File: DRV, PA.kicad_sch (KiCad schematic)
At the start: 26 parts, among them Q1 2SC5171, Q2 2SA1930, Q3 IRF630, Q4 IRF630

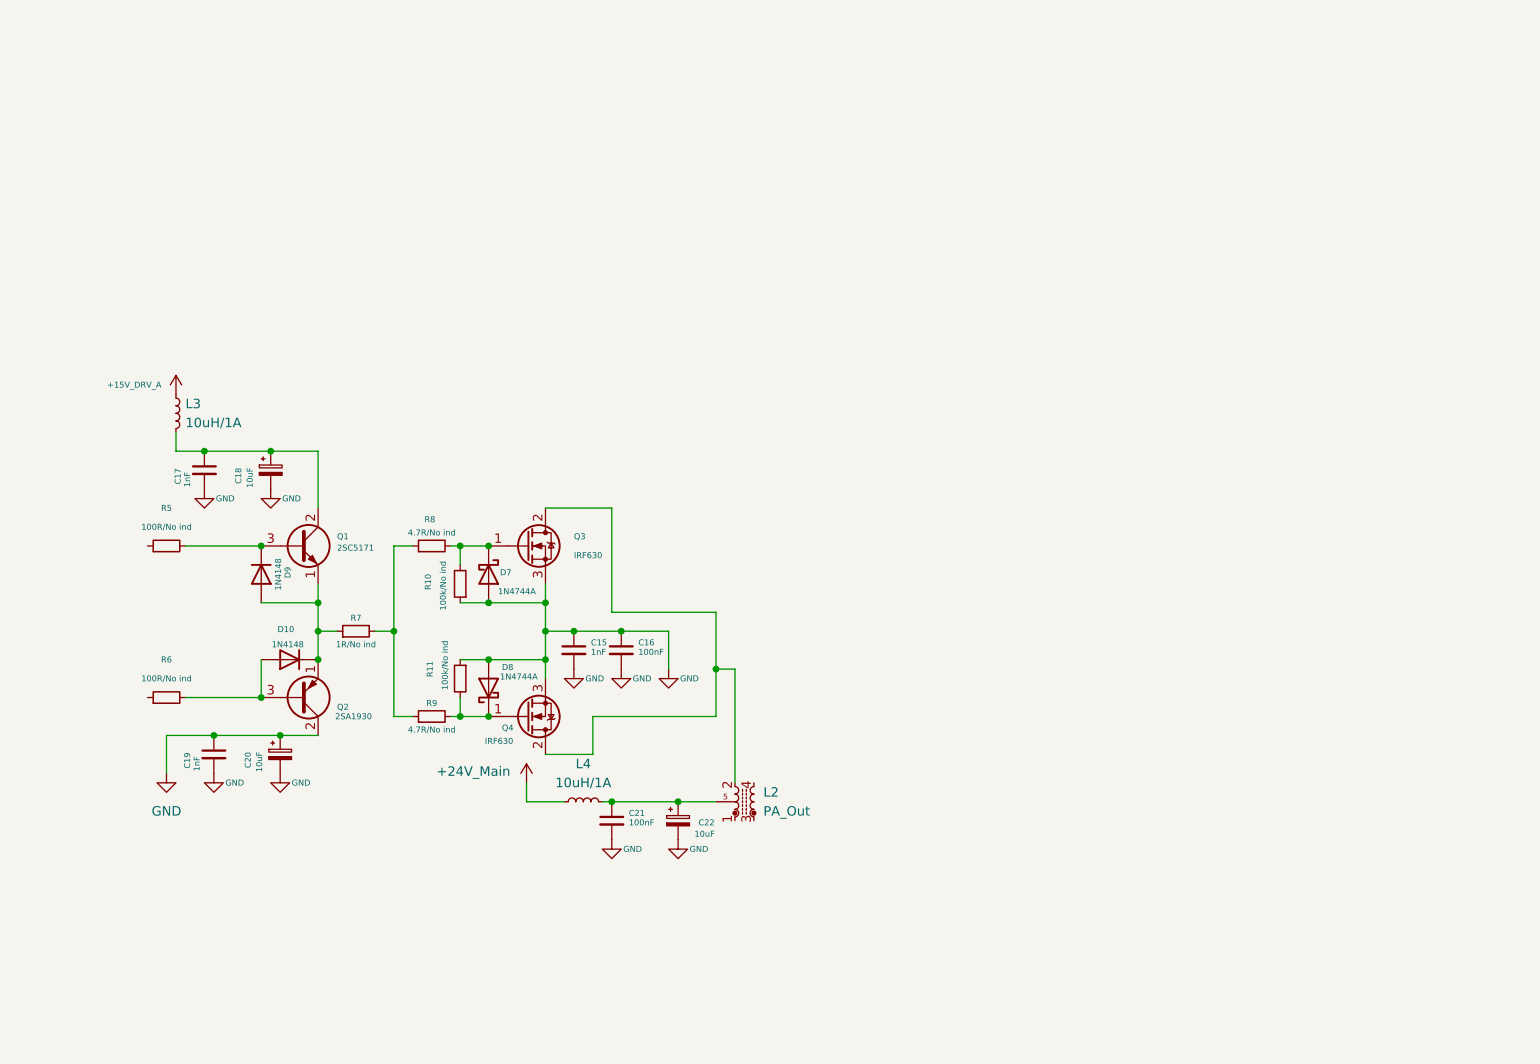
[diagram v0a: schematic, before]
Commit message: Bias Work
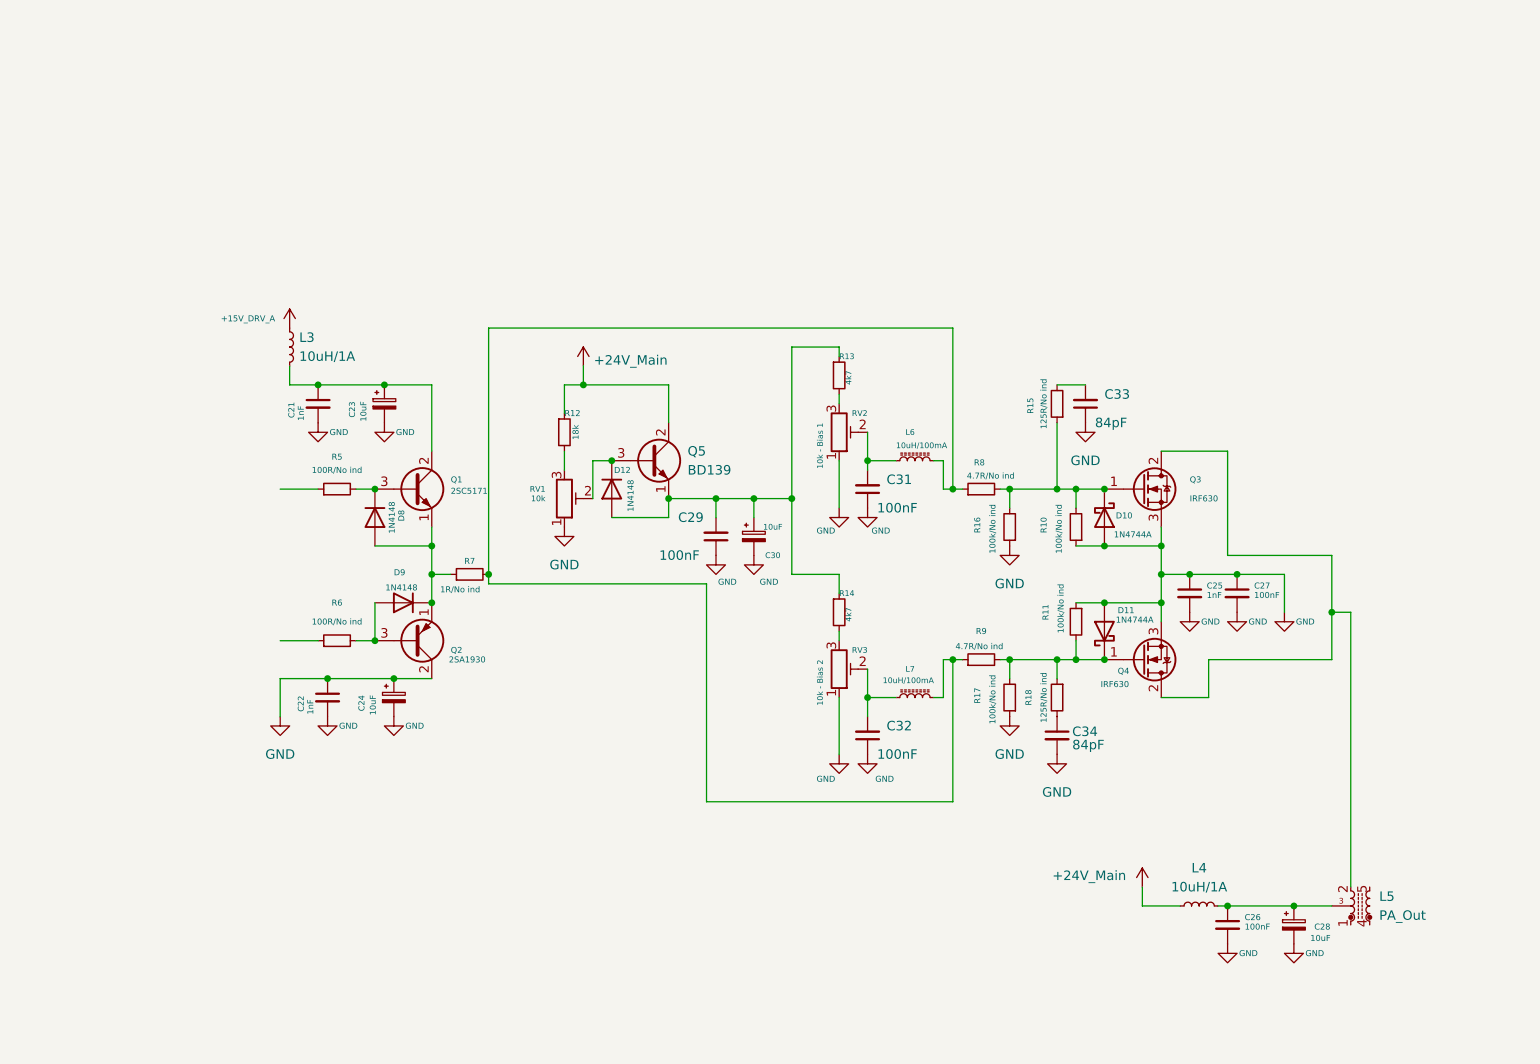
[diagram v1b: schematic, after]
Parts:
- removed L2: PA_Out, symbol Intralha.:L_Ferrite_Taped_Coupled_Small_2
- added C29, C31, C32: 100nF, symbol Device:C_Small
- added C30: 10uF, symbol Device:C_Polarized_Small
- added C33, C34: 84pF, symbol Device:C_Small
- added D12: 1N4148, Diode_THT:D_DO-35_SOD27_P7.62mm_Horizontal, symbol Diode:1N4148
- added L5: PA_Out, symbol Intralha.:L_Ferrite_Taped_Coupled_Small_2
- added L6, L7: 10uH/100mA, symbol Device:L_Ferrite_Small
- added Q5: BD139, Package_TO_SOT_THT:TO-126-3_Vertical, symbol Transistor_BJT:BD139
- added R12: 18k, symbol Device:R_Small
- added R13, R14: 4k7, symbol Device:R_Small
- added R15, R18: 125R/No ind, symbol Device:R_Small
- added R16, R17: 100k/No ind, symbol Device:R_Small
- added RV1: 10k, symbol Device:R_Potentiometer_Trim
- added RV2: 10k - Bias 1, symbol Device:R_Potentiometer_Trim
- added RV3: 10k - Bias 2, symbol Device:R_Potentiometer_Trim
- renumbered C17 to C21, C19 to C22, C18 to C23, C20 to C24, C15 to C25, C21 to C26, C16 to C27, C22 to C28, D7 to D10, D8 to D11, D9 to D8, D10 to D9
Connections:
- net +24V_Main: now also Q5.2 (C), R12.1
- net GND: now also C29.1, C30.2, C31.1, C32.1, C33.1, C34.2, R16.1, R17.1, RV1.1, RV2.1, RV3.1
- net at R7.2, R8.1, R9.1: now also L6.2, L7.2
- net at D11.1 (K), Q4.1 (G), R11.2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: now also R17.2, R18.1
- net at Q3.2 (D), Q4.2 (D): now also L5.2
- net at D10.1 (K), Q3.1 (G), R10.2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: now also R15.1, R16.2
- net at C26.1, C28.1, L4.2: now also L5.3 (Tap)
- new net: C33.2, R15.2
- new net: C29.2, C30.1, D12.2 (A), Q5.1 (E), R13.1, R14.1
- new net: R14.2, RV3.3
- new net: C31.2, L6.1, RV2.2
- new net: C32.2, L7.1, RV3.2
- new net: R13.2, RV2.3
- new net: C34.1, R18.2
- new net: D12.1 (K), Q5.3 (B), RV1.2
- new net: R12.2, RV1.3
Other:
- moved on the sheet: C21, C22, C23, C24, C25, C26, C27, C28, D10, D11, D8, D9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

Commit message: Driver bias
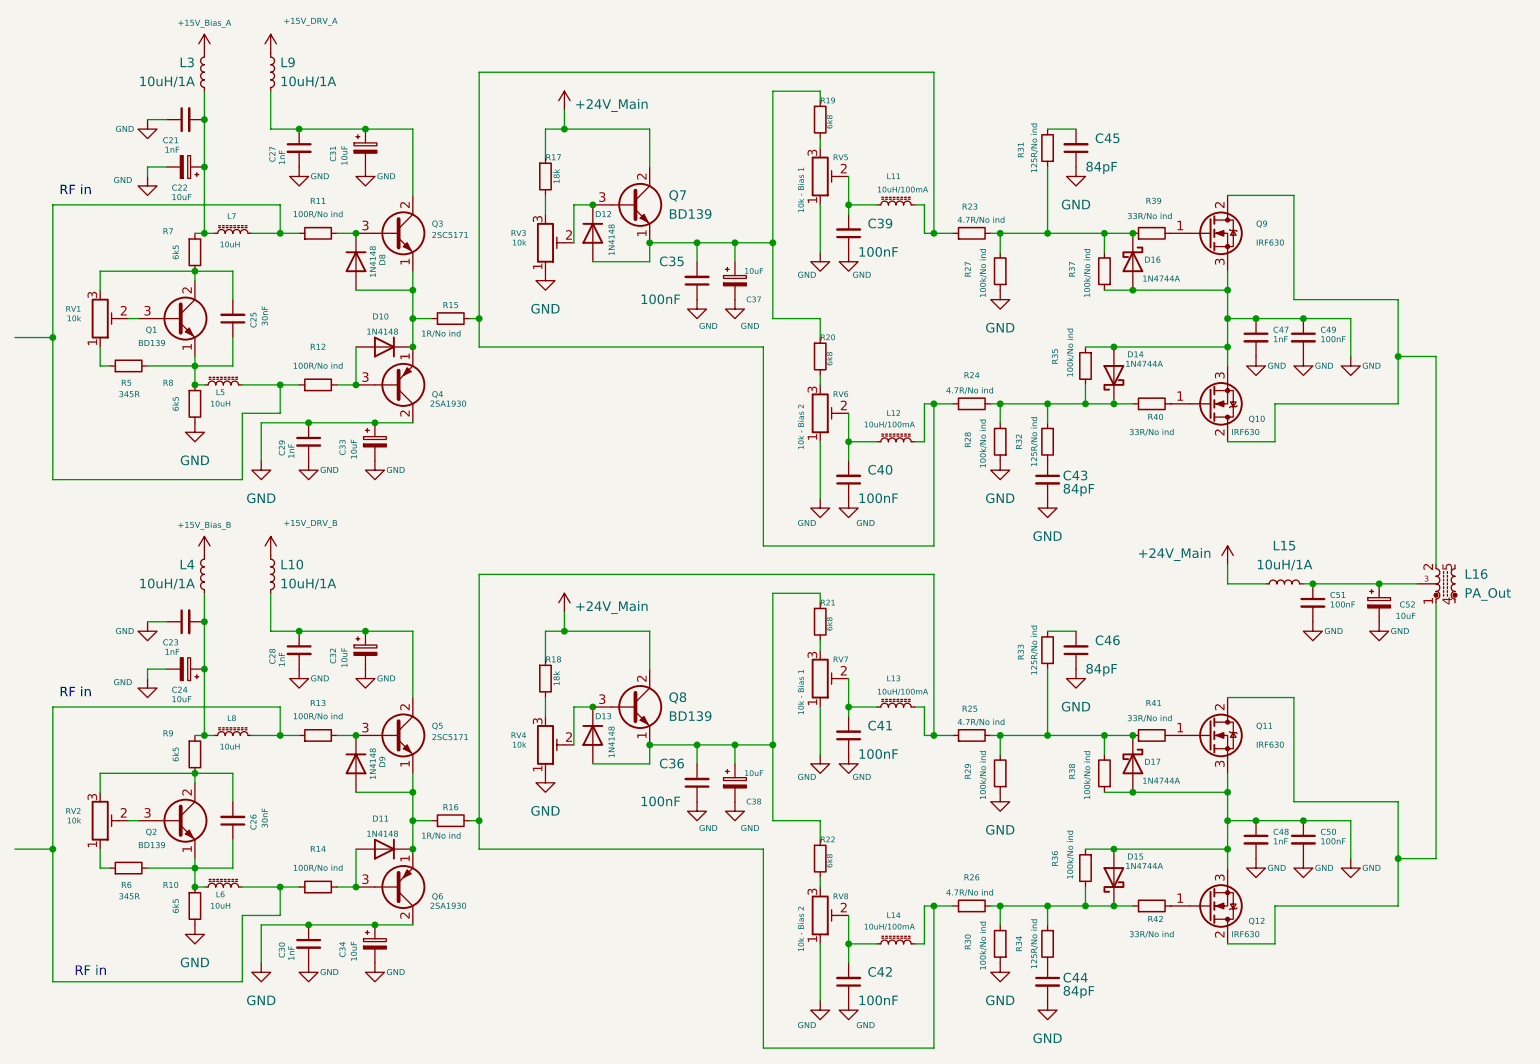
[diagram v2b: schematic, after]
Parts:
- added C21, C23, C28, C30, C48: 1nF, symbol Device:C_Small
- added C22, C24, C32, C34, C38: 10uF, symbol Device:C_Polarized_Small
- added C25, C26: 30nF, symbol Device:C_Small
- added C36, C41, C42, C50: 100nF, symbol Device:C_Small
- added C44, C46: 84pF, symbol Device:C_Small
- added D11, D13, D9: 1N4148, Diode_THT:D_DO-35_SOD27_P7.62mm_Horizontal, symbol Diode:1N4148
- added D15, D17: 1N4744A, symbol Device:D_Schottky
- added L10, L3, L4: 10uH/1A, symbol Device:L_Small
- added L13, L14: 10uH/100mA, symbol Device:L_Ferrite_Small
- added L5, L6, L7, L8: 10uH, symbol Device:L_Ferrite_Small
- added Q1, Q2, Q8: BD139, Package_TO_SOT_THT:TO-126-3_Vertical, symbol Transistor_BJT:BD139
- added Q11, Q12: IRF630, Package_TO_SOT_THT:TO-220-3_Vertical, symbol Transistor_FET:IRF540N
- added Q5: 2SC5171, Package_TO_SOT_THT:TO-126-3_Vertical, symbol Transistor_BJT:BD139
- added Q6: 2SA1930, Package_TO_SOT_THT:TO-126-3_Vertical, symbol Transistor_BJT:BD140
- added R10, R7, R8, R9: 6k5, symbol Device:R_Small
- added R13, R14: 100R/No ind, symbol Device:R_Small
- added R16: 1R/No ind, symbol Device:R_Small
- added R18: 18k, symbol Device:R_Small
- added R21, R22: 6k8, symbol Device:R_Small
- added R25, R26: 4.7R/No ind, symbol Device:R_Small
- added R29, R30, R36, R38: 100k/No ind, symbol Device:R_Small
- added R33, R34: 125R/No ind, symbol Device:R_Small
- added R39, R40, R41, R42: 33R/No ind, symbol Device:R_Small
- added R5, R6: 345R, symbol Device:R_Small
- added RV1, RV2, RV4: 10k, symbol Device:R_Potentiometer_Trim
- added RV7: 10k - Bias 1, symbol Device:R_Potentiometer_Trim
- added RV8: 10k - Bias 2, symbol Device:R_Potentiometer_Trim
- R19: renamed from R13; value 4k7 -> 6k8
- R20: renamed from R14; value 4k7 -> 6k8
- renumbered C21 to C27, C22 to C29, C23 to C31, C24 to C33, C29 to C35, C30 to C37, C31 to C39, C32 to C40, C34 to C43, C33 to C45, C25 to C47, C27 to C49, C26 to C51, C28 to C52, D9 to D10, D11 to D14, D10 to D16, L6 to L11, L7 to L12, L4 to L15, L5 to L16, L3 to L9, Q4 to Q10, Q1 to Q3, Q2 to Q4, Q5 to Q7, Q3 to Q9, R5 to R11, R6 to R12, R7 to R15, R12 to R17, R8 to R23, R9 to R24, R16 to R27, R17 to R28, R15 to R31, R18 to R32, R11 to R35, R10 to R37, RV1 to RV3, RV2 to RV5, RV3 to RV6
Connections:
- net +24V_Main: now also Q8.2 (C), R18.1
- net GND: now also C21.1, C22.2, C23.1, C24.2, C28.2, C30.1, C30.2, C32.2, C34.1, C34.2, C36.1, C38.2, C41.1, C42.1, C44.2, C46.1, C48.1, C48.2, C50.1, C50.2, D15.2 (A), D17.2 (A), Q11.3 (S), Q12.3 (S), Q6.2 (C), R10.2, R29.1, R30.1, R36.1, R38.1, R8.2, RV4.1, RV7.1, RV8.1
- net at D16.1 (K), R23.2, R27.2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: now also R39.1; no longer Q9.1 (G)
- net at D14.1 (K), R24.2, R28.2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: now also R40.1; no longer Q10.1 (G)
- net at L16.1: now also Q11.2 (D), Q12.2 (D)
- net at R11.1: now also R12.1, L5.2, L7.2
- new net: C25.1, L5.1, Q1.1 (E), R5.2, R8.1
- new net: C25.2, Q1.2 (C), R7.2, RV1.3
- new net: D17.1 (K), R25.2, R29.2, R33.1, R38.2, R41.1
- new net: C46.2, R33.2
- new net: R6.1, RV2.1
- new net: C26.1, L6.1, Q2.1 (E), R10.1, R6.2
- new net: L6.2, L8.2, R13.1, R14.1
- new net: D9.1 (K), Q5.3 (B), R13.2
- new net: D11.1 (K), D9.2 (A), Q5.1 (E), Q6.1 (E), R16.1
- new net: L13.2, L14.2, R16.2, R25.1, R26.1
- new net: C42.2, L14.1, RV8.2
- new net: C28.1, C32.1, L10.2, Q5.2 (C)
- new net: R5.1, RV1.1
- new net: Q1.3 (B), RV1.2
- new net: C26.2, Q2.2 (C), R9.2, RV2.3
- new net: Q2.3 (B), RV2.2
- new net: C44.1, R34.2
- new net: C23.2, C24.1, L4.2, L8.1, R9.1
- new net: D13.1 (K), Q8.3 (B), RV4.2
- new net: R18.2, RV4.3
- new net: D15.1 (K), R26.2, R30.2, R34.1, R36.2, R42.1
- new net: Q12.1 (G), R42.2
- new net: C21.2, C22.1, L3.2, L7.1, R7.1
- new net: R22.2, RV8.3
- new net: Q11.1 (G), R41.2
- new net: Q10.1 (G), R40.2
- new net: C36.2, C38.1, D13.2 (A), Q8.1 (E), R21.1, R22.1
- new net: C41.2, L13.1, RV7.2
- new net: R21.2, RV7.3
- new net: Q9.1 (G), R39.2
- new net: D11.2 (A), Q6.3 (B), R14.2
- new net +15V_Bias_A: L3.1
- new net +15V_Bias_B: L4.1
- new net +15V_DRV_B: L10.1
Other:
- note added: "RF in"
- moved on the sheet: C27, C29, C31, C33, C35, C37, C39, C40, C43, C45, C47, C49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
